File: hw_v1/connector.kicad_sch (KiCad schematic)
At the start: 20 parts, among them J1 Conn_02x24_Counter_Clockwise, Q3 PMN30XPX, Q4 AO3400A, U11 L78M05ABDT-TR, U12 LM74800, U19 L78M05ABDT-TR, U8 MIC5205-3.3YM5

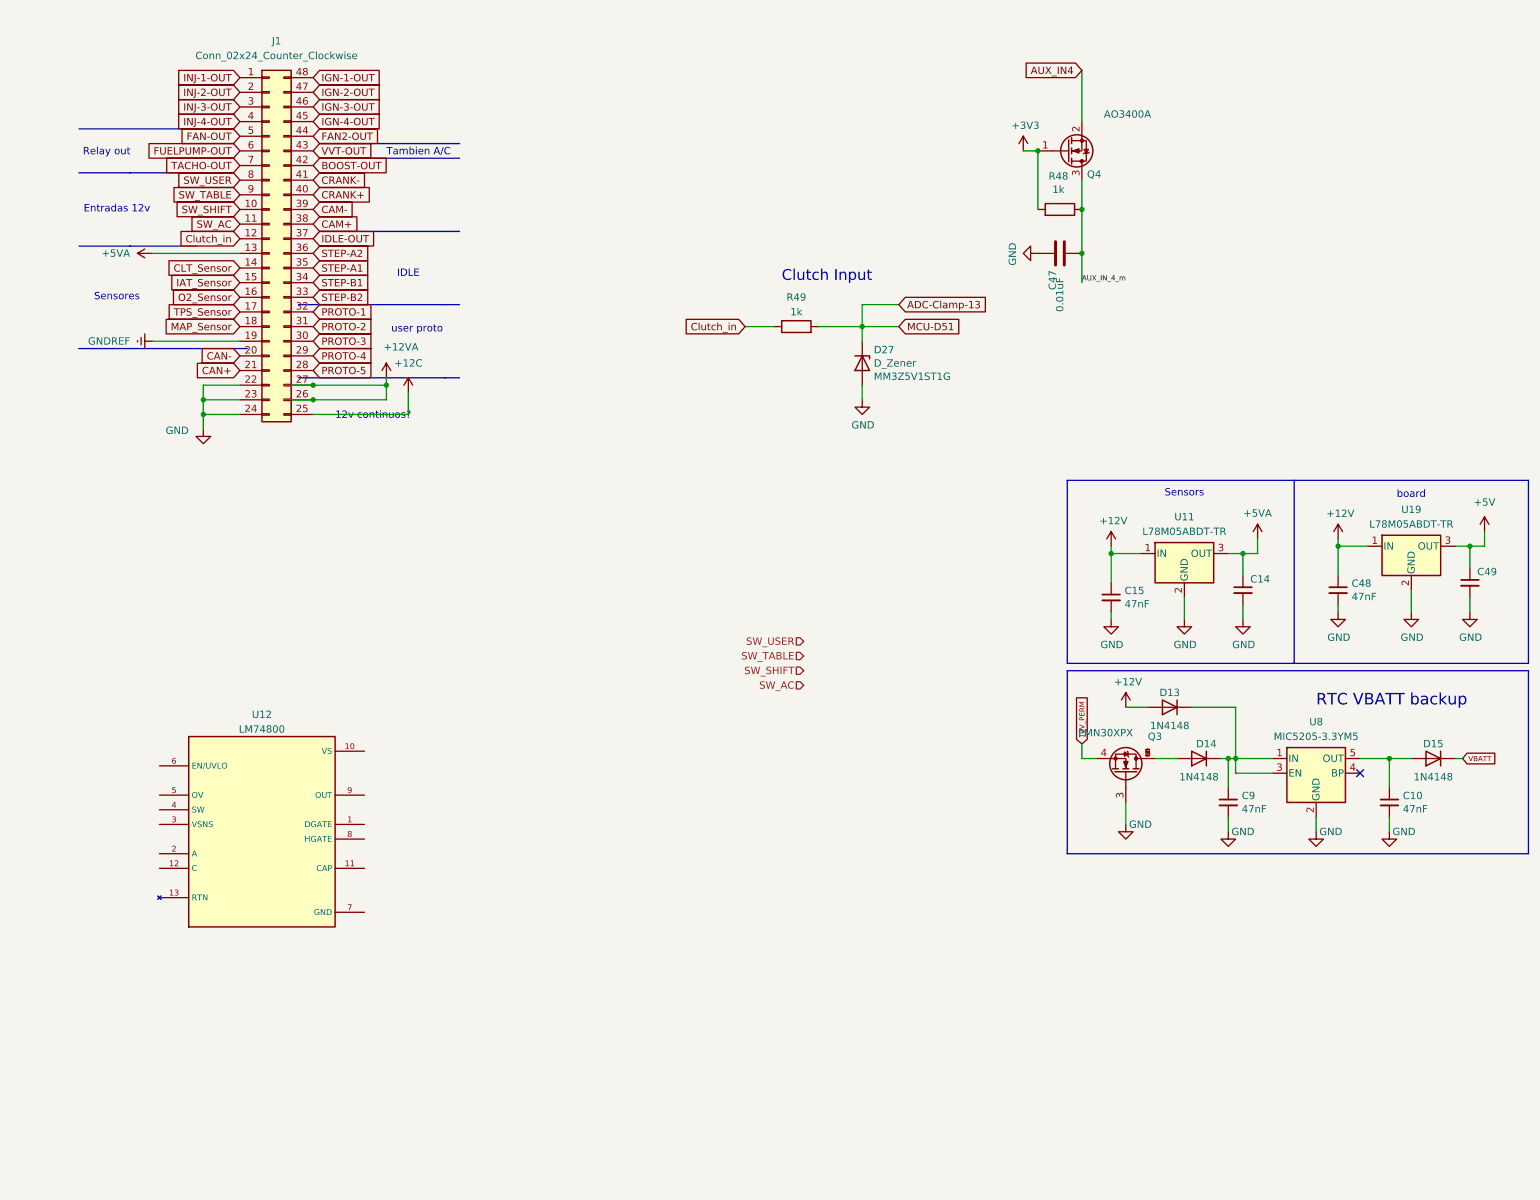
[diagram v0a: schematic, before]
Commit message: wip pcb layout
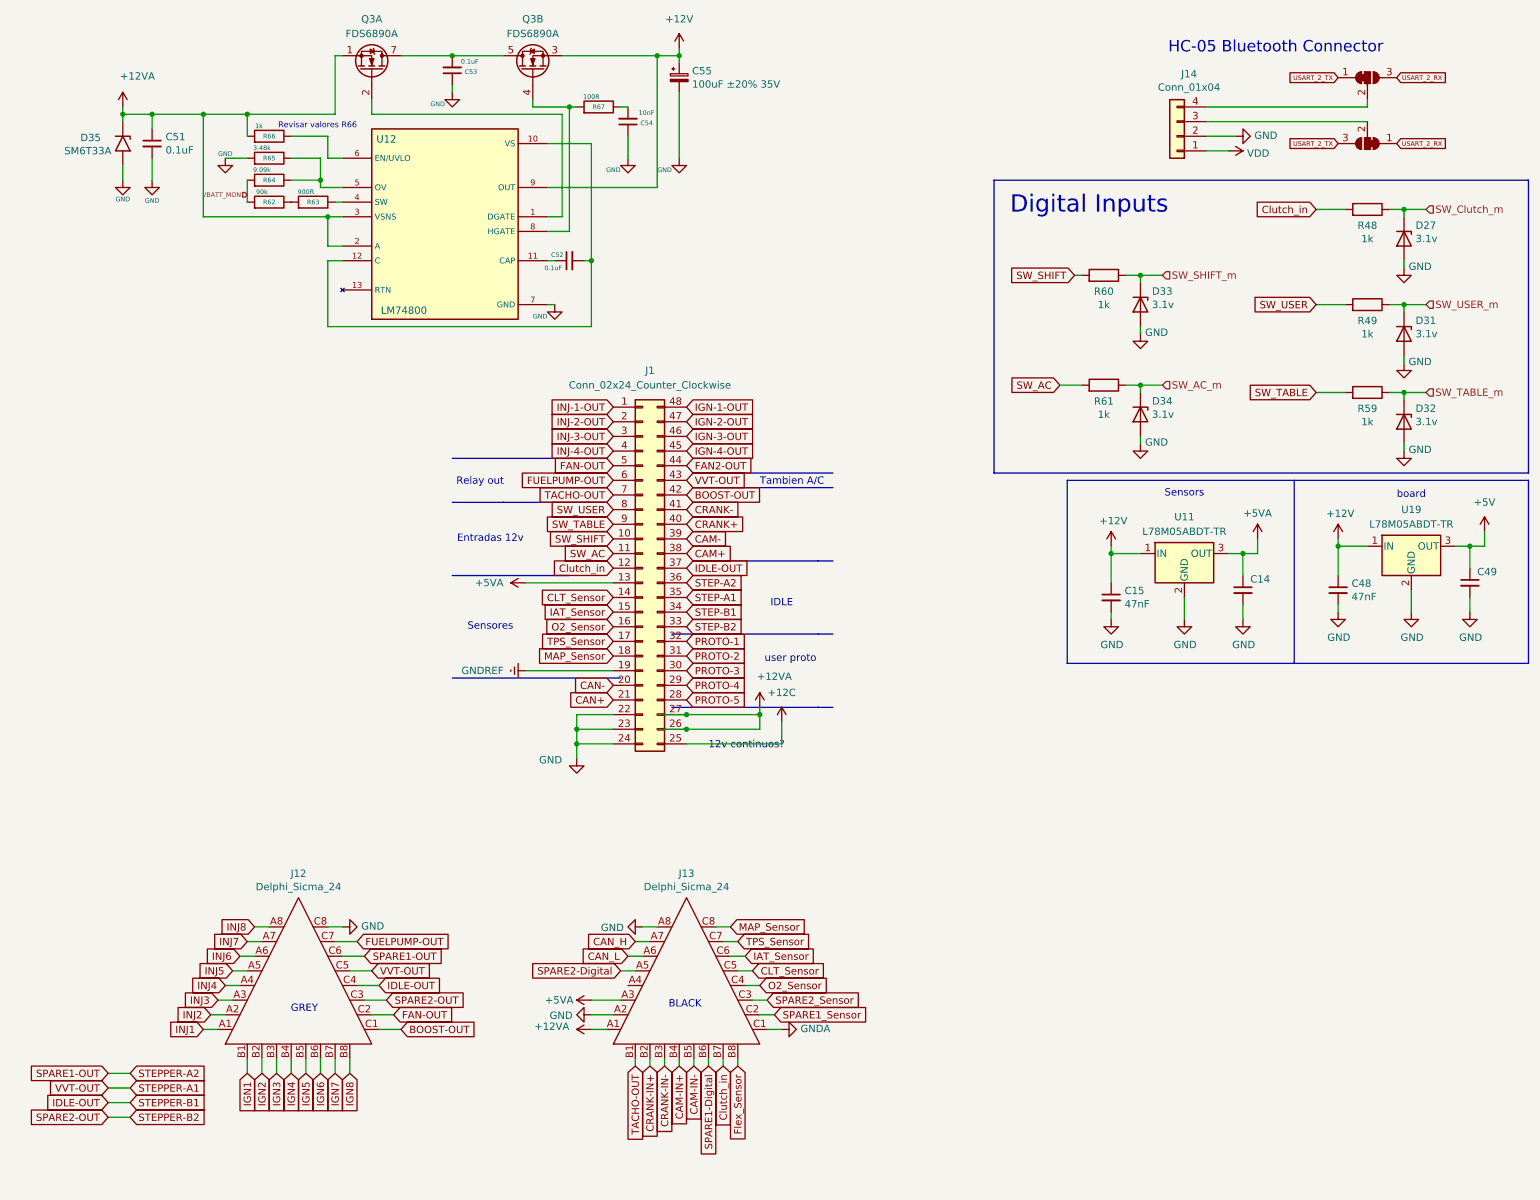
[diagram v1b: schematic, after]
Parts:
- removed C10, C9: 47nF, Capacitor_SMD:C_0603_1608Metric, symbol Device:C_Small
- removed C47: 0.01uF, Capacitor_SMD:C_0805_2012Metric, symbol Device:C
- removed D13, D14, D15: 1N4148, Diode_SMD:D_SOD-523, symbol Diode:1N4148
- removed Q3: PMN30XPX, Package_SO:TSOP-6_1.65x3.05mm_P0.95mm, symbol Transistor_FET:IRF540N
- removed Q4: AO3400A, Package_TO_SOT_SMD:SOT-23, symbol Transistor_FET:AO3400A
- removed U8: MIC5205-3.3YM5, Package_TO_SOT_SMD:SOT-23-5, symbol Regulator_Linear:MIC5205-3.3YM5
- added C51, C52, C53: 0.1uF, Capacitor_SMD:C_0805_2012Metric, symbol Device:C_Small
- added C54: 10nF, Capacitor_SMD:C_0805_2012Metric, symbol Device:C_Small
- added C55: 100uF ±20% 35V, Capacitor_SMD:CP_Elec_6.3x7.7, symbol Device:CP_Small
- added D31, D32, D33, D34: 3.1v, Diode_SMD:D_SOD-323, symbol Device:D_Zener
- added D35: SM6T33A, Diode_SMD:D_SMB, symbol Diode:SM6T33A
- added J12: Delphi_Sicma_24, uEFI_v5:Delphi_Sicma_24_Grey, symbol Connector_Automotive:Delphi_Sicma_24
- added J13: Delphi_Sicma_24, uEFI_v5:Delphi_Sicma_24_Black, symbol Connector_Automotive:Delphi_Sicma_24
- added J14: Conn_01x04, Connector_PinHeader_2.54mm:PinHeader_1x04_P2.54mm_Vertical, symbol Connector_Generic:Conn_01x04
- added JP10, JP9: SolderJumper_3_Bridged12, Jumper:SolderJumper-3_P1.3mm_Bridged2Bar12_Pad1.0x1.5mm, symbol Jumper:SolderJumper_3_Bridged12
- added Q3: FDS6890A, Package_SO:SOP-8_3.9x4.9mm_P1.27mm, symbol Transistor_FET:FDS6890A
- added R59, R60, R61, R66: 1k, Resistor_SMD:R_0603_1608Metric, symbol Device:R
- added R62: 90k, Resistor_SMD:R_0603_1608Metric, symbol Device:R
- added R63: 900R, Resistor_SMD:R_0603_1608Metric, symbol Device:R
- added R64: 9.09k, Resistor_SMD:R_0603_1608Metric, symbol Device:R
- added R65: 3.48k, Resistor_SMD:R_0603_1608Metric, symbol Device:R
- added R67: 100R, Resistor_SMD:R_0603_1608Metric, symbol Device:R
- D27: value D_Zener -> 3.1v; Digikey Part Number MM3Z5V1ST1GOSCT-ND -> (none); LCSC (none) -> C5270765; Manufacturer_Name On Semi -> (none); Manufacturer_Part_Number MM3Z5V1ST1G -> (none); Part # MM3Z5V1ST1G -> BZT52C3V3S; URL https://www.digikey.com/product-detail/en/on-semiconductor/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 -> (none)
- R49: footprint Resistor_SMD:R_0805_2012Metric -> Resistor_SMD:R_0603_1608Metric; Digikey Part Number 311-1.00KCRCT-ND -> (none); LCSC (none) -> C21190; Manufacturer_Name Yageo -> (none); Manufacturer_Part_Number RC0805FR-071KL -> (none); URL https://www.digikey.com/product-detail/en/yageo/RC0805FR-07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 -> (none)
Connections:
- net +3V3 is gone; now on net Clutch_in: R48.2
- net AUX_IN_4_m is gone; now on net SW_Clutch_m: R48.1
- net +12V: now also U12.9 (OUT), C55.1, Q3.3 (S2)
- net +12VA: now also U12.2 (A), U12.3 (VSNS), C51.1, D35.1 (A1), J13.A1, Q3.1 (S1), R66.2
- net +5VA: now also J13.A3
- net BOOST-OUT: now also J12.C1
- net CLT_Sensor: now also J13.C5
- net Clutch_in: now also J13.B7; no longer R49.1
- net FAN-OUT: now also J12.C2
- net FUELPUMP-OUT: now also J12.C7
- net GND: now also U12.7 (GND), C51.2, C53.1, C54.1, C55.2, D31.2 (A), D32.2 (A), D33.2 (A), D34.2 (A), D35.2 (A2), J12.C8, J13.A2, J13.A8, J14.2 (Pin_2), R65.2
- net IAT_Sensor: now also J13.C6
- net IDLE-OUT: now also J12.C4
- net MAP_Sensor: now also J13.C8
- net O2_Sensor: now also J13.C4
- net SW_AC: now also R61.2
- net SW_SHIFT: now also R60.2
- net SW_TABLE: now also R59.2
- net SW_USER: now also R49.2
- net TACHO-OUT: now also J13.B1
- net TPS_Sensor: now also J13.C7
- net at U12.1 (DGATE): now also Q3.2 (G1)
- net at U12.10 (VS): now also U12.12 (C), C52.2
- net at U12.11 (CAP): now also C52.1
- net at U12.4 (SW): now also R63.1
- net at U12.5 (OV): now also R64.1, R65.1
- net at U12.6 (EN/UVLO): now also R66.1
- net at U12.8 (HGATE): now also Q3.4 (G2), R67.2
- net ADC-Clamp-13 renamed SW_Clutch_m
- net SW_Clutch_m: no longer R49.2
- net VVT-OUT renamed STEPPER-A1
- net STEPPER-A1: now also J12.C5
- new net: R62.1, R63.2
- new net: C54.2, R67.1
- new net: J14.4 (Pin_4), JP9.2 (C)
- new net: C53.2, Q3.5 (D2), Q3.6 (D2), Q3.7 (D1), Q3.8 (D1)
- new net: J14.3 (Pin_3), JP10.2 (C)
- new net CAM-IN+: J13.B4
- new net CAM-IN-: J13.B5
- new net CAN_H: J13.A7
- new net CAN_L: J13.A6
- new net CRANK-IN+: J13.B2
- new net CRANK-IN-: J13.B3
- new net Flex_Sensor: J13.B8
- new net GNDA: J13.C1
- new net IGN1: J12.B1
- new net IGN2: J12.B2
- new net IGN3: J12.B3
- new net IGN4: J12.B4
- new net IGN5: J12.B5
- new net IGN6: J12.B6
- new net IGN7: J12.B7
- new net IGN8: J12.B8
- new net INJ1: J12.A1
- new net INJ2: J12.A2
- new net INJ3: J12.A3
- new net INJ4: J12.A4
- new net INJ5: J12.A5
- new net INJ6: J12.A6
- new net INJ7: J12.A7
- new net INJ8: J12.A8
- new net SPARE1-Digital: J13.B6
- new net SPARE1-OUT: J12.C6
- new net SPARE1_Sensor: J13.C2
- new net SPARE2-Digital: J13.A5
- new net SPARE2-OUT: J12.C3
- new net SPARE2_Sensor: J13.C3
- new net SW_AC_m: D34.1 (K), R61.1
- new net SW_SHIFT_m: D33.1 (K), R60.1
- new net SW_TABLE_m: D32.1 (K), R59.1
- new net SW_USER_m: D31.1 (K), R49.1
- new net USART_2_RX: JP10.1 (A), JP9.3 (B)
- new net USART_2_TX: JP10.3 (B), JP9.1 (A)
- new net VBATT_MON: R62.2, R64.2
- new net VDD: J14.1 (Pin_1)
- no-connect marks 1 -> 0
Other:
- note added: "BLACK"
- note added: "Digital Inputs"
- note added: "GREY"
- note added: "HC-05 Bluetooth Connector"
- note added: "Revisar valores R66"
- note removed: "Clutch Input"
- note removed: "RTC VBATT backup"
- moved on the sheet: D27, J1, R48, U12
